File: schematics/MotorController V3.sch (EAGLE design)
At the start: 54 parts, among them IC1 7805, Q1 BC307

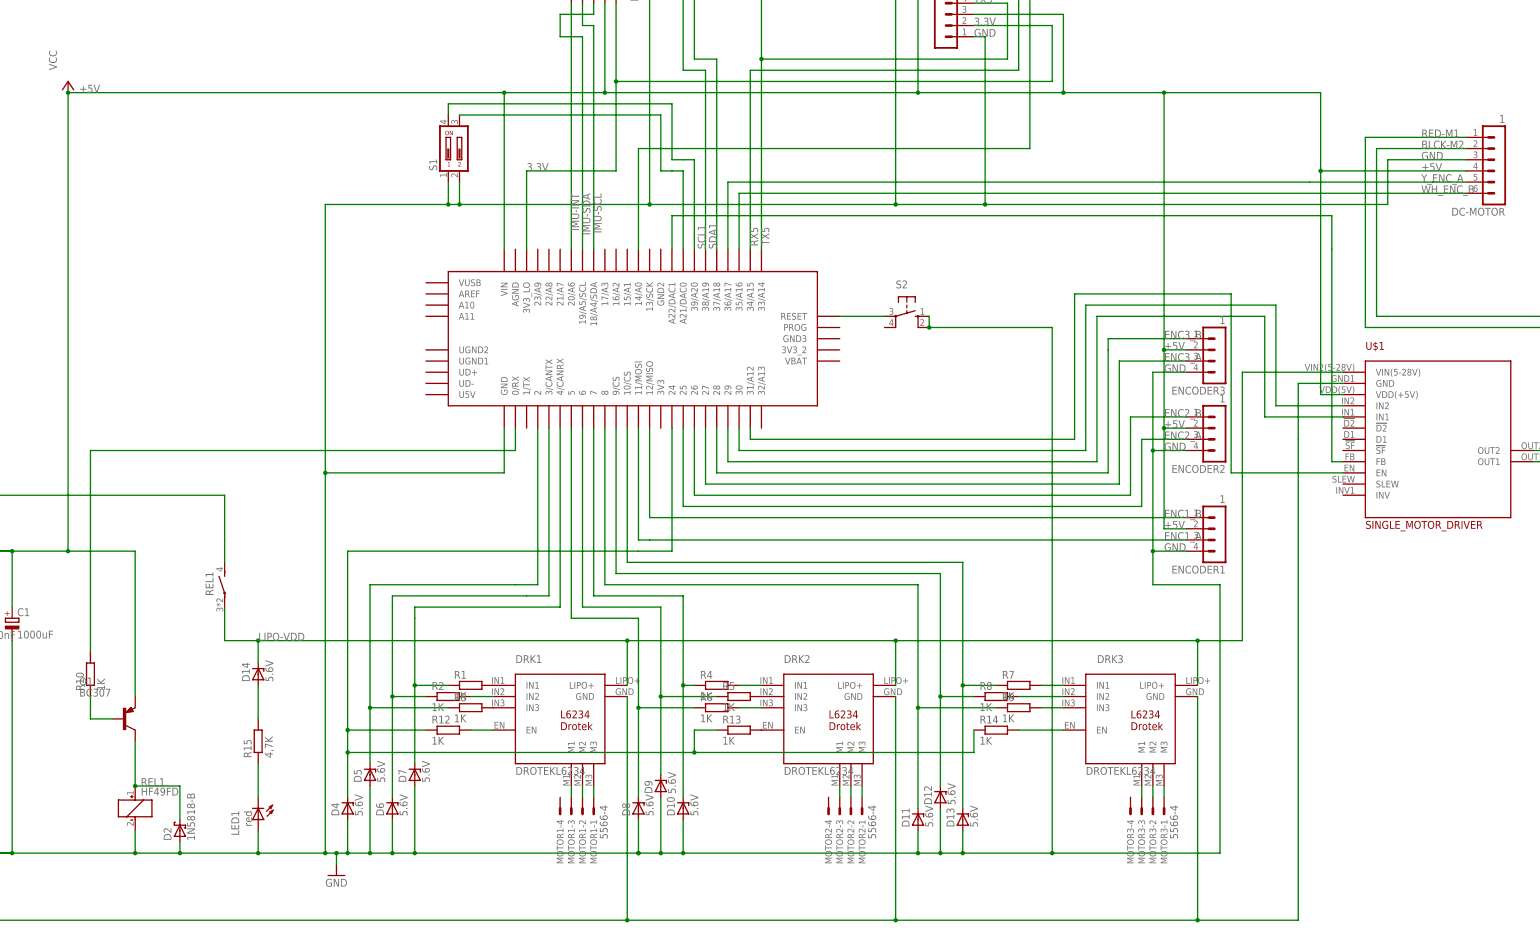
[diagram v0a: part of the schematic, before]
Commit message: no message
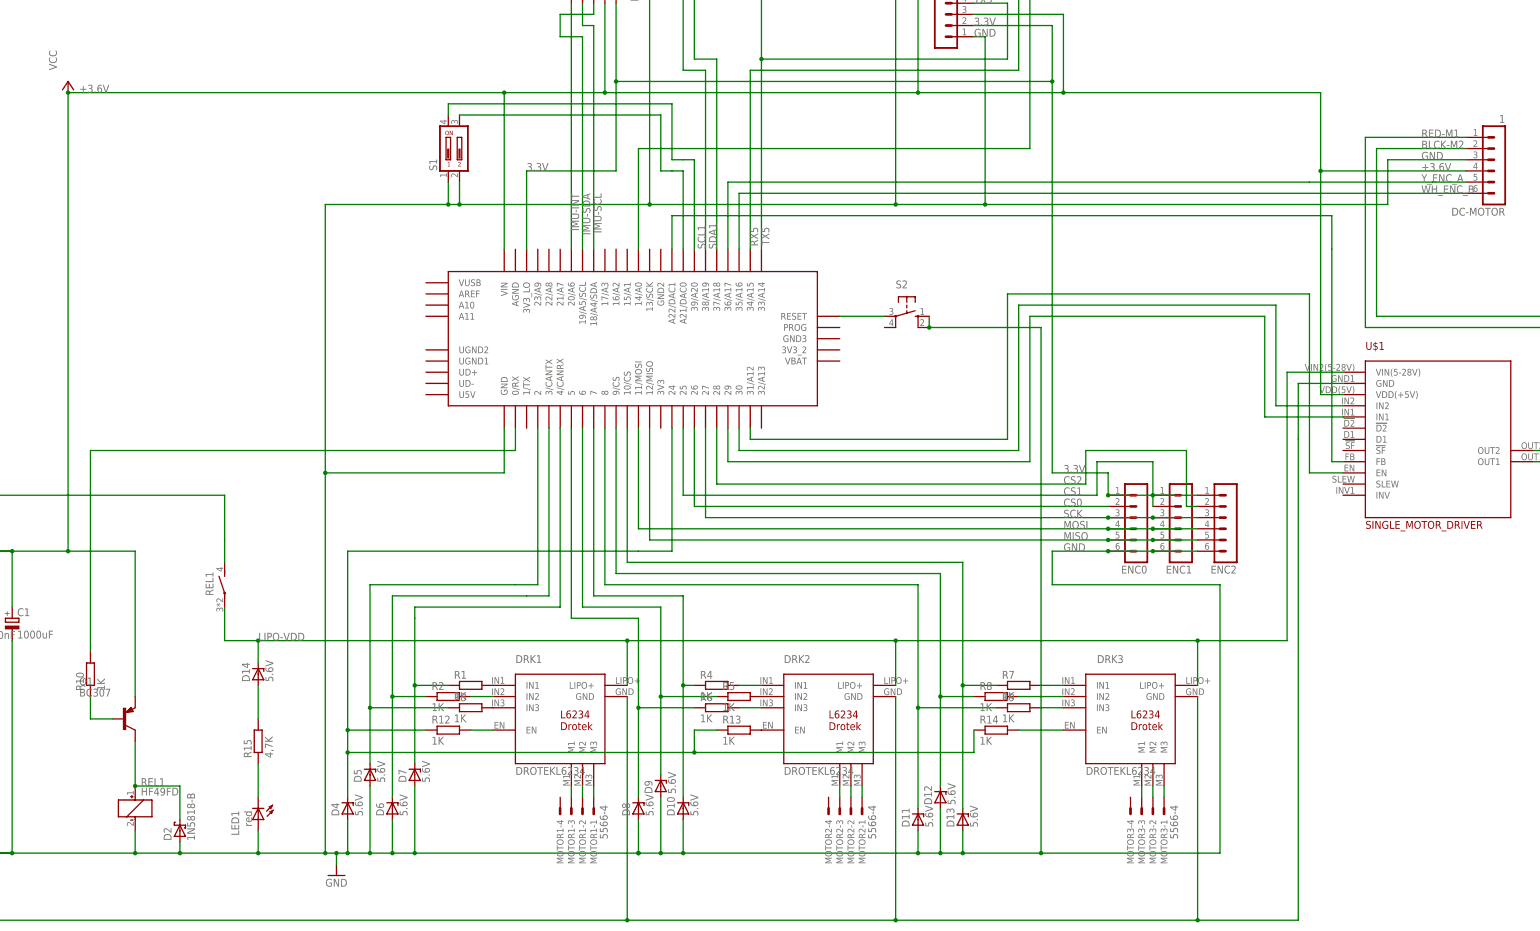
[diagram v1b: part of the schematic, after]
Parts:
- removed ENCODER1, ENCODER2, ENCODER3: 1, con-lstb:MA04-1
- added ENC0, ENC1, ENC2: (no value), con-lstb:MA06-1
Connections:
- removed net +5V: C1.+, C3.1, CONTROL.3, D3.A, DC-MOTOR.4, ENCODER1.2, ENCODER2.2, ENCODER3.2, IC1.OUT, IMU-I2C.4, PRJ1.VIN, Q1.E, U$1.VDD(+5V), U$2.D0
- removed net ENC1_A: ENCODER1.3, PRJ1.11/MOSI
- removed net ENC1_B: ENCODER1.1, PRJ1.12/MISO
- removed net ENC2_A: ENCODER2.3, PRJ1.25
- removed net ENC2_B: ENCODER2.1, PRJ1.26
- removed net ENC3_A: ENCODER3.3, PRJ1.27
- removed net ENC3_B: ENCODER3.1, PRJ1.28
- new net +3.6V: C1.+, C3.1, CONTROL.3, D3.A, DC-MOTOR.4, IC1.OUT, IMU-I2C.4, PRJ1.VIN, Q1.E, U$1.VDD(+5V), U$2.D0
- new net CS0: ENC0.2, PRJ1.26
- new net CS1: ENC1.2, PRJ1.25
- new net CS2: ENC2.2, PRJ1.28
- new net MISO: ENC0.5, ENC1.5, ENC2.5, PRJ1.12/MISO
- new net MOSI: ENC0.4, ENC1.4, ENC2.4, PRJ1.11/MOSI
- new net SCK: ENC0.3, ENC1.3, ENC2.3, PRJ1.27
- net 3.3V: now also ENC0.1, ENC1.1, ENC2.1
- net GND: now also ENC0.6, ENC1.6, ENC2.6; no longer ENCODER1.4, ENCODER2.4, ENCODER3.4
